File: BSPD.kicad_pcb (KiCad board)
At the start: 2 copper layers, 148.6 x 83.8 mm, 62 parts, among them J1 Conn_01x03, J2 Conn_01x03, J3 Conn_01x03, J4 Screw_Terminal_01x02, K1 MCCMA51-S-DC12V-C, Q1 IRLZ44Z, U1 4011, U10 LM2901, U11 4012, U12 74LS573, U13 4040, U14 4040, U15 4040, U16 L7805, U2 4011, U3 4011, U4 4011, U5 4011, U6 4011, U7 4011, U8 4011, U9 LM2901, X1 ASZKDV-32.768KHz

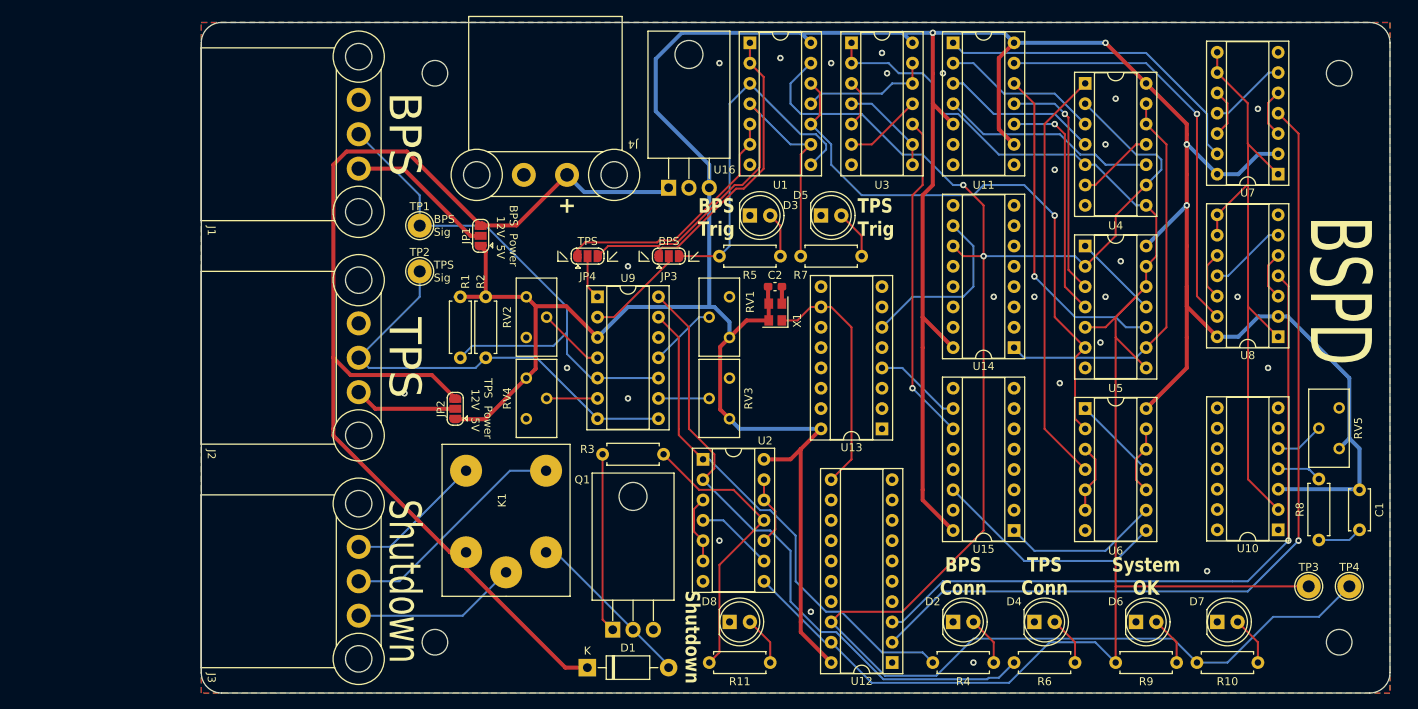
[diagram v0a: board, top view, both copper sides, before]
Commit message: Complete new version
Signed-off-by: Oliver Gaskell <og305@cam.ac.uk>
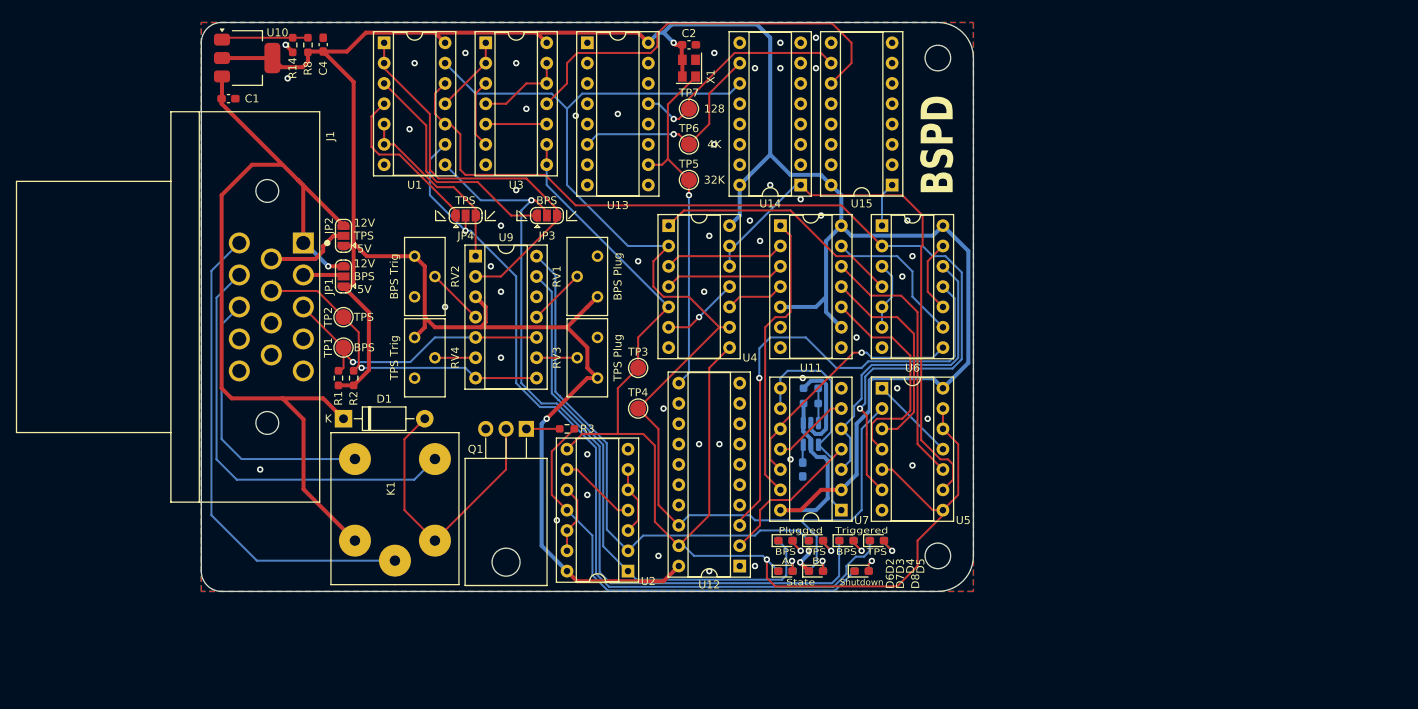
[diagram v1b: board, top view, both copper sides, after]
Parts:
- removed J2, J3: Conn_01x03, BSPD_footprints:ATF13-3P-BM03
- removed J4: Screw_Terminal_01x02, BSPD_footprints:ATF13-2P-BM03
- removed MNT3, MNT4: MountingHole_3.2mm_M3, MountingHole:MountingHole_3.2mm_M3
- removed RV5: R_Potentiometer, Potentiometer_THT:Potentiometer_Bourns_3296Y_Vertical
- removed U16: L7805, Package_TO_SOT_THT:TO-220-3_Horizontal_TabDown
- removed U8: 4011, Package_DIP:DIP-14_W7.62mm_Socket
- added C3: 200n, Capacitor_SMD:C_0603_1608Metric_Pad1.08x0.95mm_HandSolder, B.Cu at (127.3, 78.7)
- added C4: 1u, Capacitor_SMD:C_0603_1608Metric_Pad1.08x0.95mm_HandSolder, F.Cu at (67.3, 25.6)
- added R12: 750k, Resistor_SMD:R_0603_1608Metric_Pad0.98x0.95mm_HandSolder, B.Cu at (128.3, 70.5)
- added R13: 100k, Resistor_SMD:R_0603_1608Metric_Pad0.98x0.95mm_HandSolder, B.Cu at (128.3, 68.6)
- added R14: 715, Resistor_SMD:R_0603_1608Metric_Pad0.98x0.95mm_HandSolder, F.Cu at (63.5, 25.7)
- added TP5: TestPoint, TestPoint:TestPoint_Pad_D2.0mm, F.Cu at (113.0, 42.5)
- added TP6: TestPoint, TestPoint:TestPoint_Pad_D2.0mm, F.Cu at (113.0, 38.1)
- added TP7: TestPoint, TestPoint:TestPoint_Pad_D2.0mm, F.Cu at (113.0, 33.7)
- added U17: MAX6895, Package_TO_SOT_SMD:SOT-23-6_Handsoldering, B.Cu at (128.3, 74.3)
- C1: value 100n -> 0.1u; footprint Capacitor_THT:C_Disc_D5.0mm_W2.5mm_P5.00mm -> Capacitor_SMD:C_0603_1608Metric_Pad1.08x0.95mm_HandSolder
- D2, D3, D4, D5, D6, D7, D8: footprint LED_THT:LED_D5.0mm -> LED_SMD:LED_0603_1608Metric_Pad1.05x0.95mm_HandSolder
- J1: value Conn_01x03 -> Conn_01x14; footprint BSPD_footprints:ATF13-3P-BM03 -> FBR_Footprints:TE_776267-1
- R1, R2: value 5K -> 100K; footprint Resistor_THT:R_Axial_DIN0207_L6.3mm_D2.5mm_P7.62mm_Horizontal -> Resistor_SMD:R_0603_1608Metric_Pad0.98x0.95mm_HandSolder
- R10, R11, R4, R5, R6, R7, R9: value 220R -> 180; footprint Resistor_THT:R_Axial_DIN0207_L6.3mm_D2.5mm_P7.62mm_Horizontal -> Resistor_SMD:R_0603_1608Metric_Pad0.98x0.95mm_HandSolder; moved to B.Cu
- R3: footprint Resistor_THT:R_Axial_DIN0207_L6.3mm_D2.5mm_P7.62mm_Horizontal -> Resistor_SMD:R_0603_1608Metric_Pad0.98x0.95mm_HandSolder
- R8: value 1M -> 240; footprint Resistor_THT:R_Axial_DIN0207_L6.3mm_D2.5mm_P7.62mm_Horizontal -> Resistor_SMD:R_0603_1608Metric_Pad0.98x0.95mm_HandSolder
- TP1, TP2, TP3, TP4: footprint TestPoint:TestPoint_THTPad_D3.0mm_Drill1.5mm -> TestPoint:TestPoint_Pad_D2.0mm
- U10: value LM2901 -> LM317_SOT-223; footprint Package_DIP:DIP-14_W7.62mm_Socket -> Package_TO_SOT_SMD:SOT-223-3_TabPin2
- U9: value LM2901 -> TLC3704
- moved C1 149.6 mm to (55.5, 32.4), turned to 0 degrees
- moved U10 141.7 mm to (57.8, 27.3), turned to 0 degrees
- moved R8 140.7 mm to (65.4, 25.7)
- moved TP4 91.6 mm to (106.7, 71.1)
- moved TP3 88.2 mm to (106.7, 66.0)
- moved U7 68.9 mm to (132.1, 83.8)
- moved U13 60.7 mm to (100.3, 25.4), turned to 0 degrees
- moved R10 56.4 mm to (128.9, 91.4)
- moved U4 55.0 mm to (110.5, 48.3)
- moved MNT2 51.3 mm to (144.1, 89.5)
- moved D7 50.6 mm to (128.9, 91.4)
- moved R9 50.2 mm to (125.1, 91.4)
- moved MNT1 50.2 mm to (144.1, 27.3)
- moved G*** 47.8 mm to (144.8, 41.9)
- moved U15 45.8 mm to (138.4, 43.2)
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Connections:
- C1 pad 1: +5V -> +12V
- C1 pad 2: Net-(C1-Pad2) -> GND
- J1 pad 1: GND -> +12V
- J1 pad 2: /BPS_Sig -> /BPS_Power
- J1 pad 3: /BPS_Power -> /BPS_Sig
- JP3 pad 2: Net-(JP3-C) -> /BPS_Trig
- JP3 pad 3: /BPS_Trig -> Net-(JP3-B)
- JP4 pad 2: Net-(JP4-C) -> /TPS_Trig
- JP4 pad 3: /TPS_Trig -> Net-(JP4-B)
- R5 pad 2: /BPS_Trig -> /TPS_Plugged
- R6 pad 2: /TPS_Plugged -> /BPS_Trig
- R8 pad 1: Net-(C1-Pad2) -> +5V
- R8 pad 2: Net-(U10A--) -> Net-(U10-ADJ)
- U1 pad 1: Net-(JP3-A) -> Net-(JP3-B)
- U1 pad 2: Net-(JP3-A) -> Net-(JP3-B)
- U1 pad 3: /BPS_Trig -> Net-(JP3-A)
- U1 pad 4: /TPS_Trig -> Net-(JP4-A)
- U1 pad 5: Net-(JP4-A) -> Net-(JP4-B)
- U1 pad 6: Net-(JP4-A) -> Net-(JP4-B)
- U10 pad 1: unconnected-(U10-Pad1) -> Net-(U10-ADJ)
- U10 pad 2: /RST -> +5V
- U10 pad 3: +5V -> +12V
- U13 pad 13: unconnected-(U13-Q7-Pad13) -> /State Machine/Timers/128CLK
- U13 pad 4: /State Machine/Timers/256CLK -> unconnected-(U13-Q6-Pad4)
- U15 pad 1: Net-(U15-Q11) -> /State Machine/10T
- U15 pad 10: /State Machine/Timers/256CLK -> /State Machine/Timers/128CLK
- U15 pad 14: Net-(U15-Q9) -> unconnected-(U15-Q9-Pad14)
- U3 pad 1: /SM_Ok -> Net-(U1-Pad11)
- U3 pad 10: /State Machine/Timers/Reset_Counting -> Net-(U3-Pad10)
- U3 pad 11: Net-(U3-Pad11) -> /State Machine/Timers/Reset_Counting
- U3 pad 12: Net-(U1-Pad11) -> Net-(U3-Pad12)
- U3 pad 13: Net-(U1-Pad11) -> Net-(U3-Pad12)
- U3 pad 2: /SM_Ok -> Net-(U1-Pad11)
- U3 pad 4: Net-(U3-Pad4) -> Net-(U3-Pad12)
- U3 pad 5: Net-(U3-Pad3) -> Net-(U3-Pad10)
- U3 pad 6: Net-(U3-Pad11) -> Net-(U3-Pad3)
- U3 pad 8: Net-(U3-Pad4) -> /SM_Ok
- U3 pad 9: Net-(U3-Pad4) -> /SM_Ok
- U6 pad 11: /State Machine/10T -> Net-(U12-D1)
- U6 pad 12: Net-(U6-Pad10) -> Net-(U6-Pad12)
- U6 pad 8: Net-(U15-Q9) -> Net-(U6-Pad8)
- U6 pad 9: Net-(U15-Q11) -> Net-(U11-Pad13)
- U7 pad 10: Net-(U7-Pad10) -> Net-(U6-Pad8)
- U7 pad 12: Net-(U7-Pad10) -> Net-(U6-Pad8)
- U7 pad 3: Net-(U7-Pad3) -> Net-(U6-Pad12)
- U7 pad 5: Net-(U7-Pad3) -> Net-(U6-Pad12)
- U9 pad 1: Net-(JP4-C) -> Net-(JP4-B)
- U9 pad 2: Net-(JP3-C) -> Net-(JP3-B)
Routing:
- net Net-(U12-D0): track 110.5 -> 18.8 mm, vias 1 -> 0
- net +5V: track 448.5 -> 385.7 mm, vias 4 -> 2
- net /State Machine/State_B: track 221.9 -> 160.0 mm, vias 2 -> 0
- net /BPS_Trig: track 44.2 -> 103.1 mm, vias 0 -> 1
- net Net-(JP3-B): track 0.00 -> 50.7 mm
- net /RST: track 78.9 -> 29.1 mm
- net /TPS_Trig: track 57.5 -> 105.1 mm, vias 0 -> 1
- net /System_OK: track 73.1 -> 120.4 mm
- net /ShutdownC: track 20.7 -> 60.8 mm
- net Net-(U6-Pad12): track 0.00 -> 39.0 mm
- net +12V: track 146.3 -> 111.1 mm, vias 0 -> 1
- net /BPS_Sig: track 70.4 -> 37.0 mm, vias 0 -> 1
- net Net-(U11-Pad13): track 51.9 -> 18.8 mm, vias 1 -> 0
- net Net-(U6-Pad8): track 0.00 -> 31.4 mm, vias 0 -> 1
- net /SM_Ok: track 197.8 -> 167.3 mm, vias 0 -> 1
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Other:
- board size 148.6 x 83.8 mm -> 96.5 x 71.1 mm
- board text added: "128"
- board text added: "12V BPS 5V"
- board text added: "12V TPS 5V"
- board text added: "32K"
- board text added: "4K"
- board text added: "A"
- board text added: "B"
- board text added: "BPS Plug"
- board text added: "Designed by Oliver Gaskell, Dec 2024"
- board text added: "Plugged"
- board text added: "State"
- board text added: "TPS Plug"
- board text added: "Triggered"
- board text removed: "+"
- board text removed: "12V GND"
- board text removed: "BPS Conn"
- board text removed: "BPS Power 12V 5V"
- board text removed: "BPS Sig"
- board text removed: "Designed by Oliver Gaskell"
- board text removed: "System OK"
- board text removed: "TPS Conn"
- board text removed: "TPS Power 12V 5V"
- board text removed: "TPS Sig"
